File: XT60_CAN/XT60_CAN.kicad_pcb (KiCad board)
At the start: 2 copper layers, 132.1 x 68.6 mm, 40 parts, among them J1 XT60_IN, J10 +12v, J15 XT60_CH4, J16 XT60_CH5, J2 XT60_CH1, J3 +5v, J4 +9v, J5 +12v, J6 +5v, J7 +9v, J8 XT60_CH2, J9 XT60_CH3, U1 MP1584, U2 MP1584, U3 MP1584

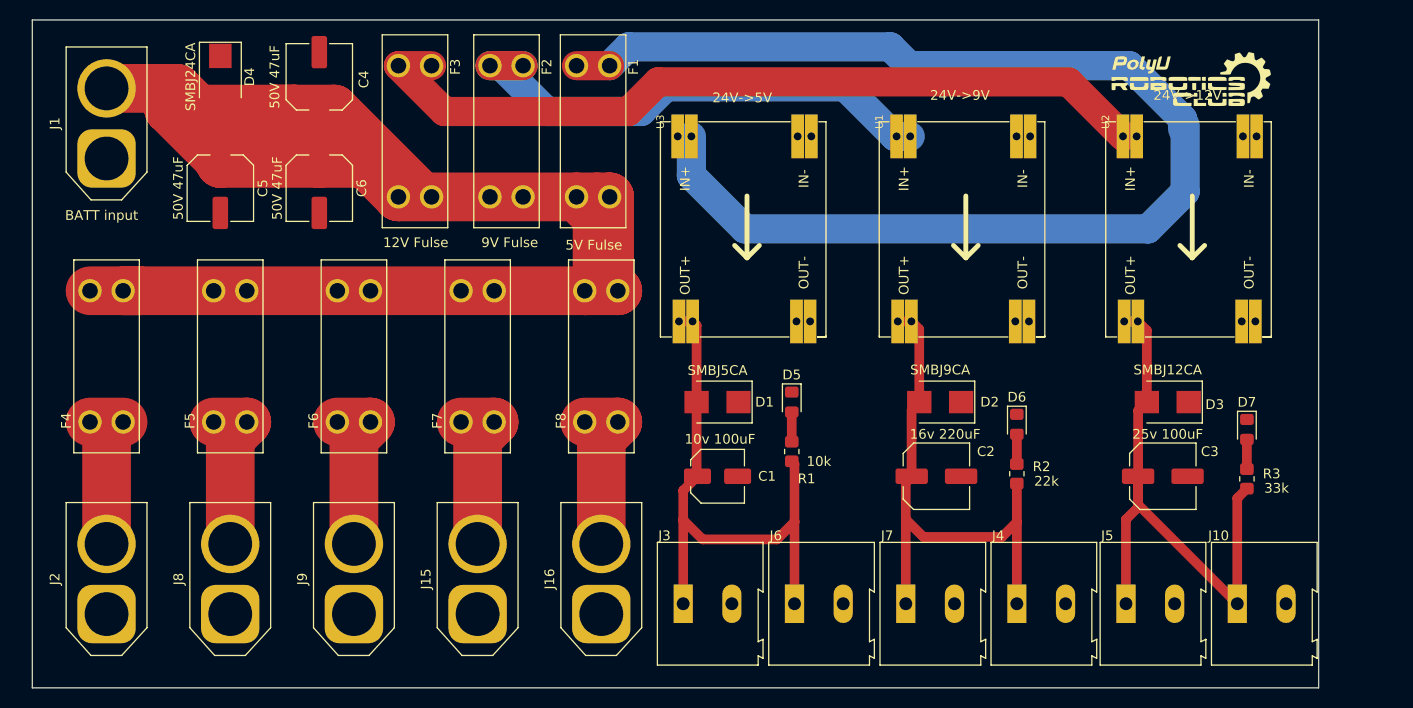
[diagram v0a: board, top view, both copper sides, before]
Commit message: terminal
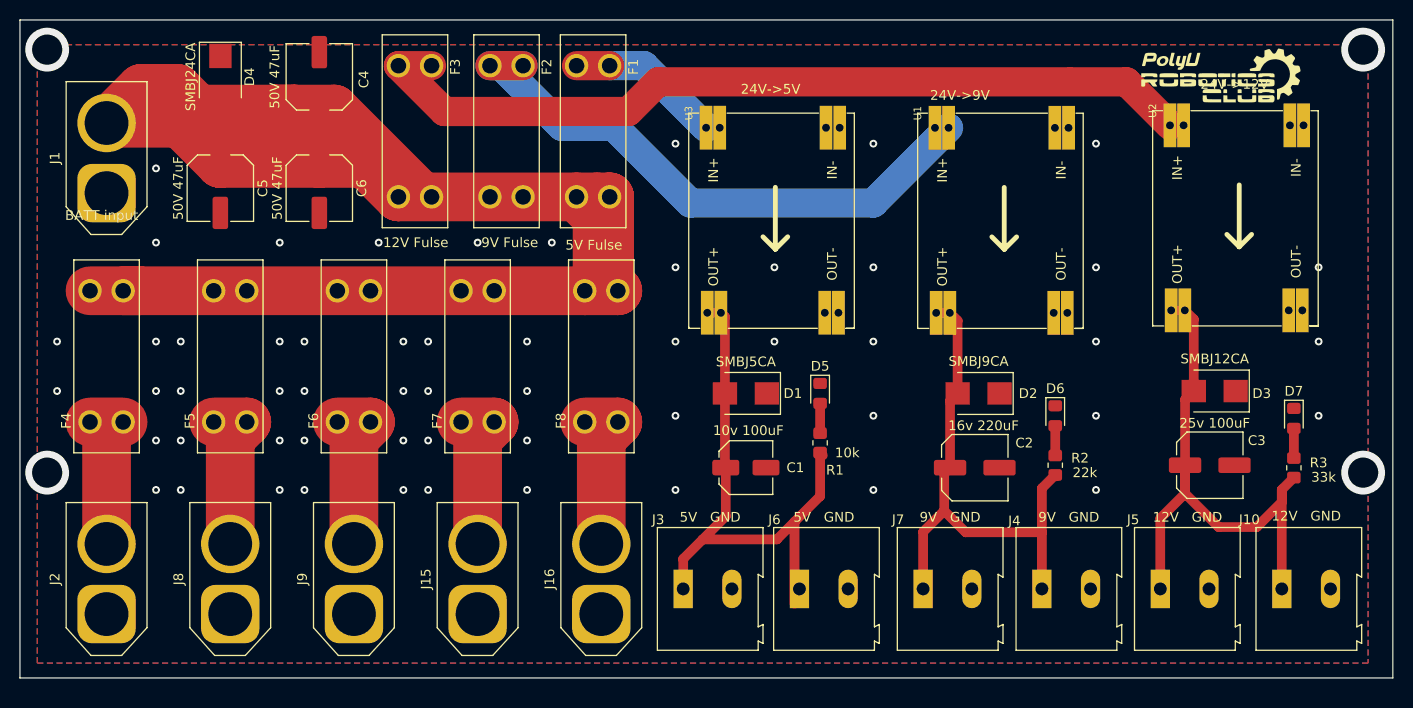
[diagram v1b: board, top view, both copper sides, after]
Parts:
- added G***: LOGO, PolyuRobotics:Club_logo, B.Cu at (158.8, 62.2)
- moved R3 4.95 mm to (188.0, 68.8)
- moved D7 4.95 mm to (188.0, 63.8)
- moved C3 4.95 mm to (179.3, 68.6)
- moved D3 4.95 mm to (179.8, 61.0)
- moved U2 4.95 mm to (173.5, 32.2)
- moved J10 4.82 mm to (186.7, 81.3)
- moved D2 4.04 mm to (155.6, 61.2)
- moved D6 4.04 mm to (163.5, 63.5)
- moved R2 4.04 mm to (163.5, 68.6)
- moved U1 4.04 mm to (149.3, 32.4)
- moved C2 4.04 mm to (155.2, 68.8)
- moved J5 3.84 mm to (174.2, 81.3)
- moved J1 3.56 mm to (66.0, 40.6)
- moved G*** 3.07 mm to (180.6, 28.8)
- moved D1 3.04 mm to (131.7, 61.2)
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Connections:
- J1 pad 1: GNDPWR -> GND
- J15 pad 1: GNDPWR -> GND
- J16 pad 1: GNDPWR -> GND
- J2 pad 1: GNDPWR -> GND
- J8 pad 1: GNDPWR -> GND
- J9 pad 1: GNDPWR -> GND
- U1 pad IN1-: GNDPWR -> GND
- U1 pad IN2-: GNDPWR -> GND
- U1 pad OUT1-: GNDPWR -> GND
- U1 pad OUT2-: GNDPWR -> GND
- U2 pad IN1-: GNDPWR -> GND
- U2 pad IN2-: GNDPWR -> GND
- U2 pad OUT1-: GNDPWR -> GND
- U2 pad OUT2-: GNDPWR -> GND
- U3 pad IN1-: GNDPWR -> GND
- U3 pad IN2-: GNDPWR -> GND
- U3 pad OUT1-: GNDPWR -> GND
- U3 pad OUT2-: GNDPWR -> GND
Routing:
- net Net-(F1-Pad1): track 132.5 -> 15.9 mm
- net +24V: track 199.8 -> 225.5 mm
- net Net-(F2-Pad1): track 53.4 -> 61.3 mm
- net Net-(F3-Pad1): track 83.2 -> 87.4 mm
- net +9V: track 56.6 -> 55.0 mm
- net +12V: track 61.3 -> 60.7 mm
- net GND: vias 0 -> 56
- net (no net): vias 0 -> 4
- added copper zone on B.Cu, net GND
- added copper zone on F.Cu, net GND
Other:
- board size 132.1 x 68.6 mm -> 141 x 67.6 mm
- board text added: "12V GND"
- board text added: "5V GND"
- board text added: "9V GND"
